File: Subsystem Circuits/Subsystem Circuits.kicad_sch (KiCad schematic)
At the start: 0 parts

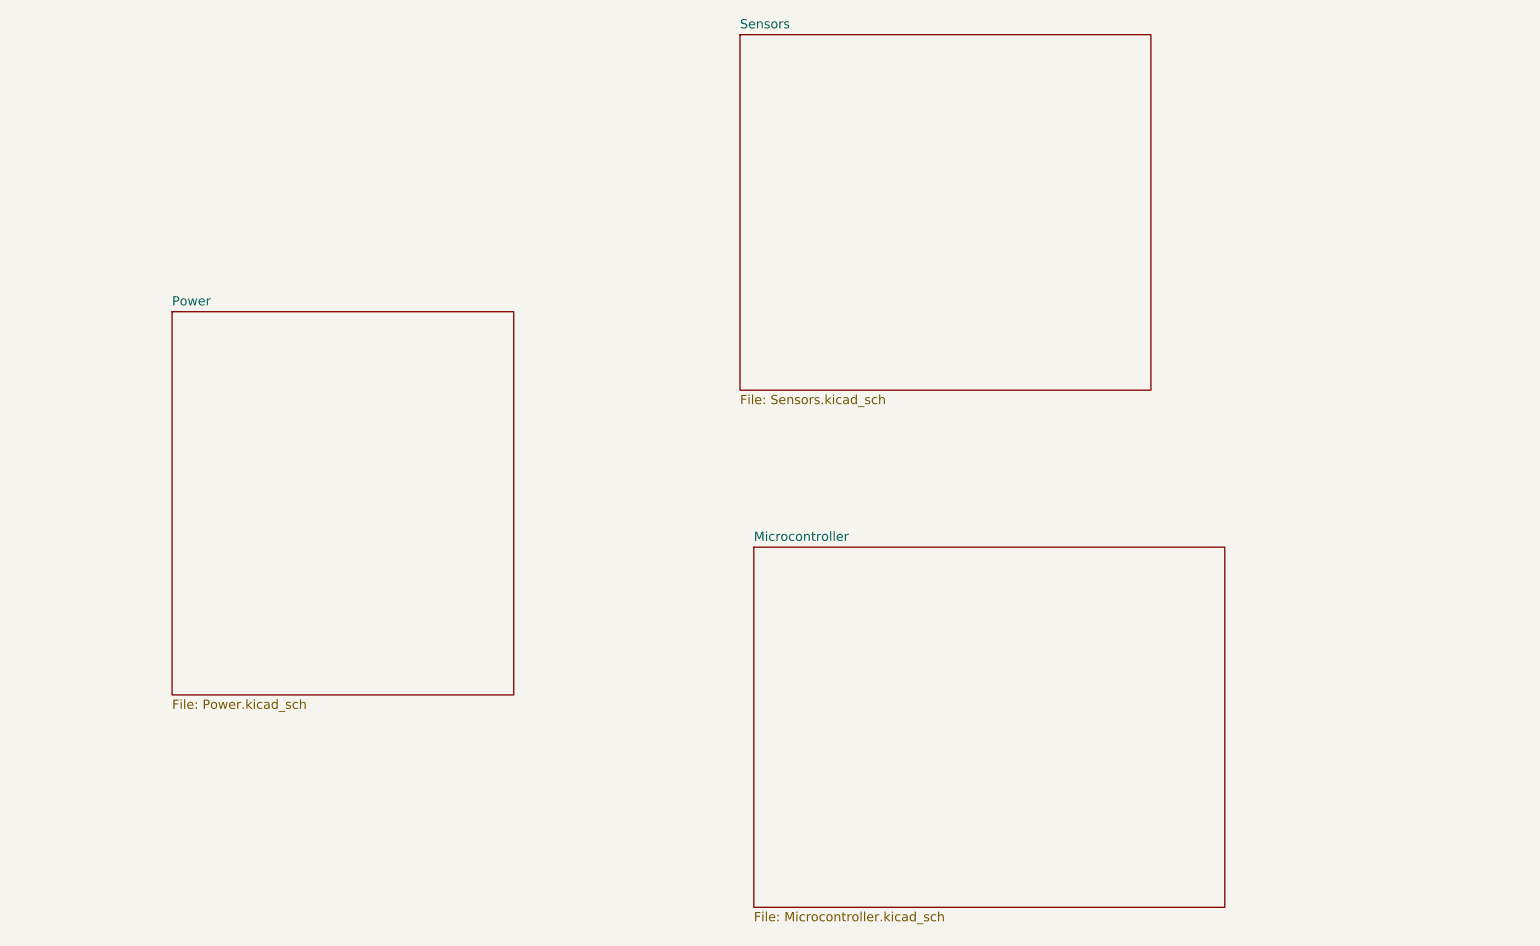
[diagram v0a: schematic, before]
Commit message: stuff
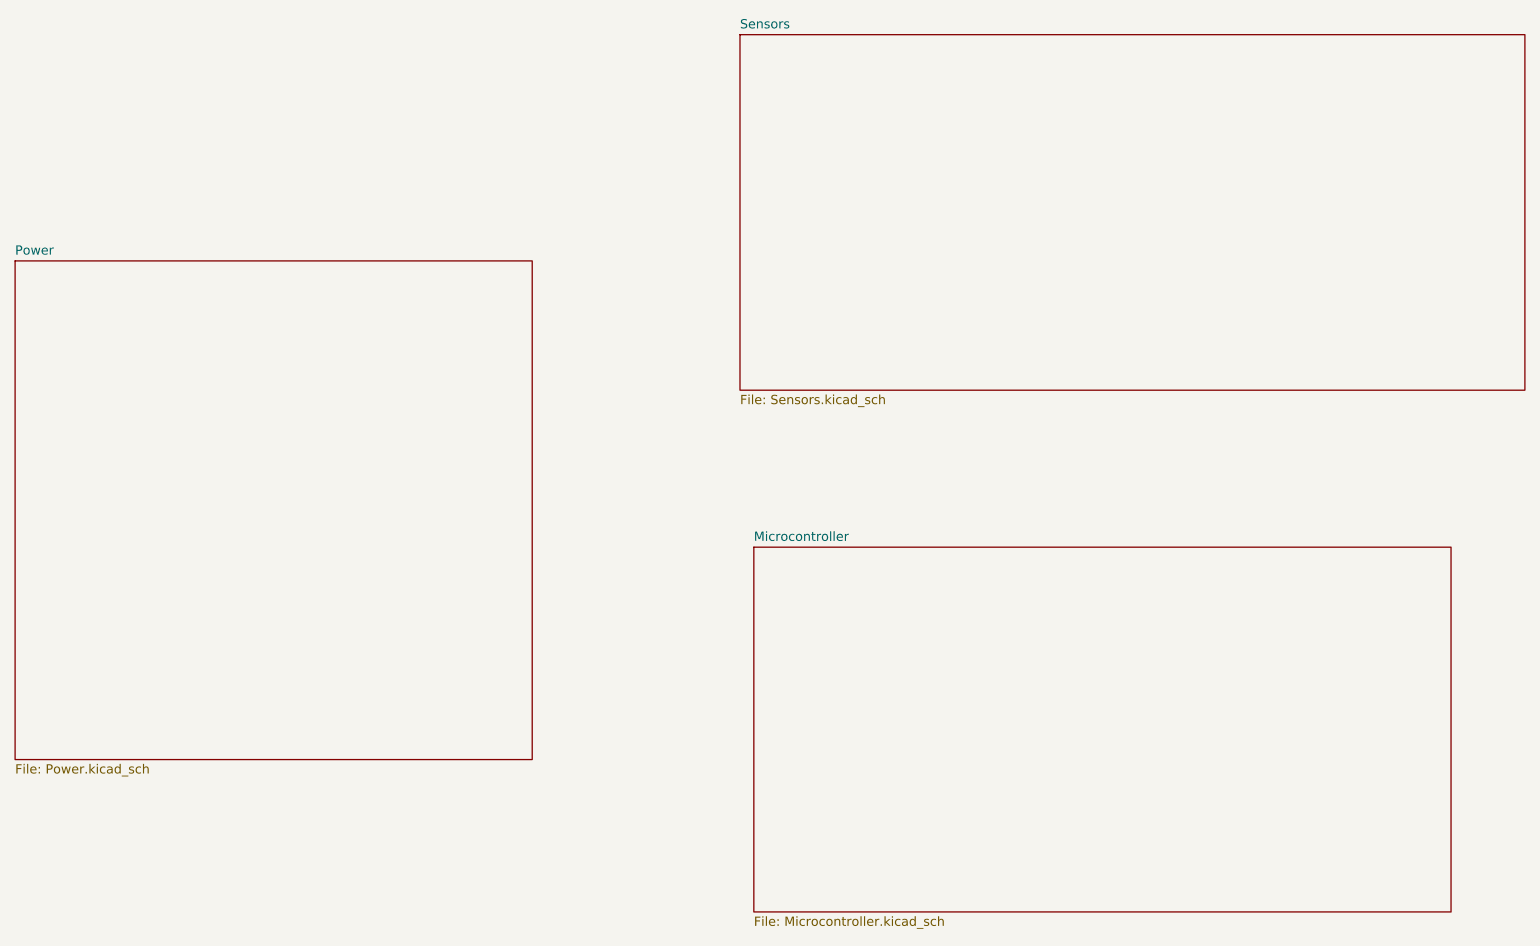
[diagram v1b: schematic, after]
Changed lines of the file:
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@@
 	(paper "A4")
 	(sheet
-		(at 46.355 69.85)
-		(size 46.99 52.705)
+		(at 24.765 62.865)
+		(size 71.12 68.58)
 		(fields_autoplaced yes)
 		(stroke
@@
 		)
 		(property "Sheetname" "Power"
-			(at 46.355 69.1384 0)
+			(at 24.765 62.1534 0)
 			(effects
 				(font
@@
 		)
 		(property "Sheetfile" "Power.kicad_sch"
-			(at 46.355 123.1396 0)
+			(at 24.765 132.0296 0)
 			(effects
 				(font
@@
 	(sheet
 		(at 126.365 102.235)
-		(size 64.77 49.53)
+		(size 95.885 50.165)
 		(fields_autoplaced yes)
 		(stroke
@@
 		)
 		(property "Sheetfile" "Microcontroller.kicad_sch"
-			(at 126.365 152.3496 0)
+			(at 126.365 152.9846 0)
 			(effects
 				(font
@@
 	(sheet
 		(at 124.46 31.75)
-		(size 56.515 48.895)
+		(size 107.95 48.895)
 		(fields_autoplaced yes)
 		(stroke
